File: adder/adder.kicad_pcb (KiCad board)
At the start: 2 copper layers, 52.9 x 21.5 mm, 29 parts

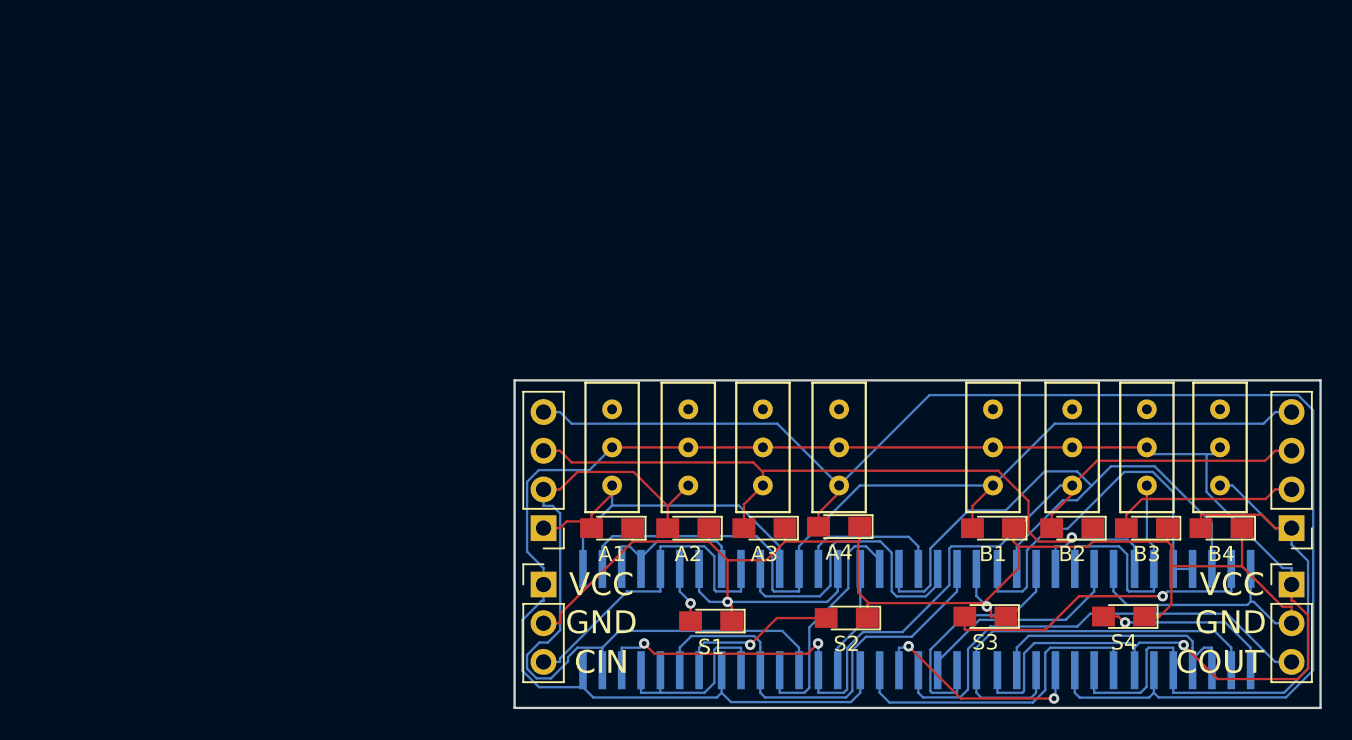
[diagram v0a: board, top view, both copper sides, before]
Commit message: Started on adder v3
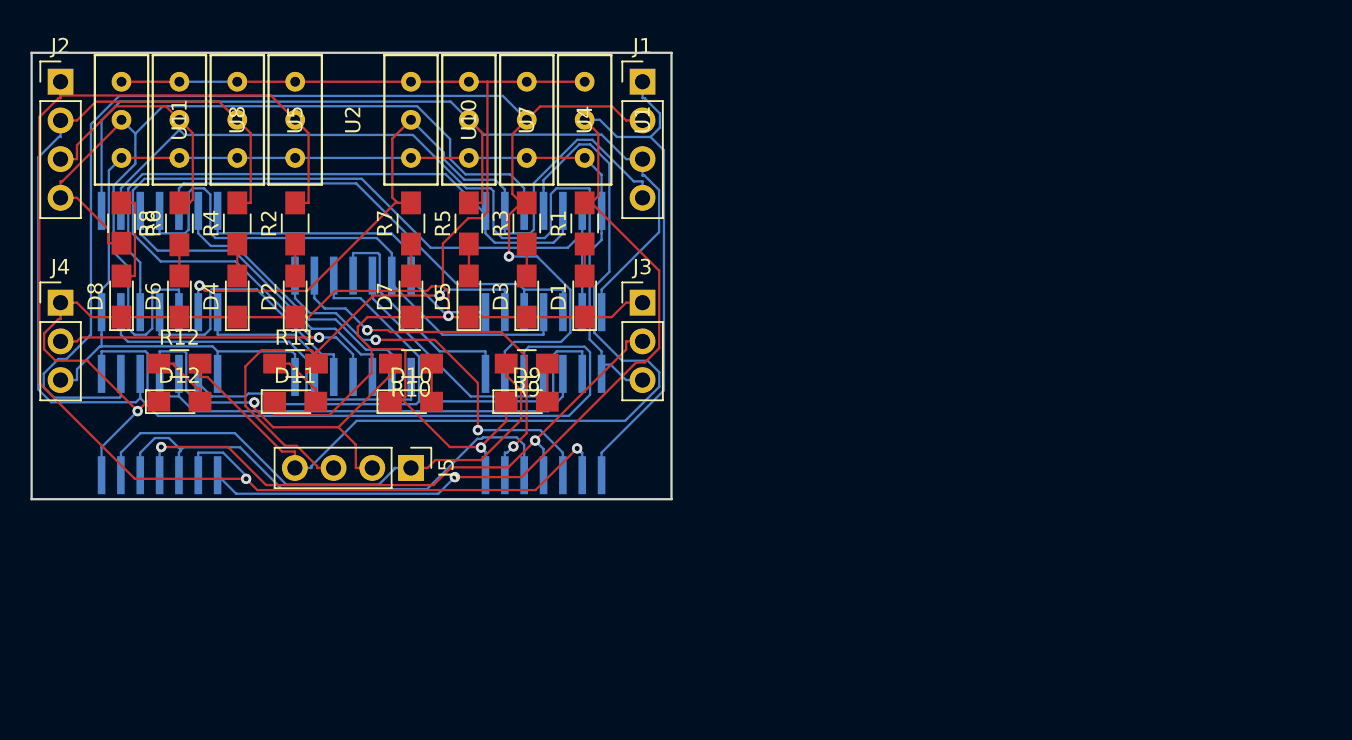
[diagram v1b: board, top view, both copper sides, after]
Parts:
- removed A1: LA1, LEDs:LED_0805_HandSoldering
- removed A1: A1, library:mini-vertical-slide-switch
- removed A2: LA2, LEDs:LED_0805_HandSoldering
- removed A2: A2, library:mini-vertical-slide-switch
- removed A3: LA3, LEDs:LED_0805_HandSoldering
- removed A3: A3, library:mini-vertical-slide-switch
- removed A4: A4, LEDs:LED_0805_HandSoldering
- removed A4: A4, library:mini-vertical-slide-switch
- removed AND (x2): AND, library:ssop14
- removed B1: LB1, LEDs:LED_0805_HandSoldering
- removed B1: B1, library:mini-vertical-slide-switch
- removed B2: LB2, LEDs:LED_0805_HandSoldering
- removed B2: B2, library:mini-vertical-slide-switch
- removed B3: LB3, LEDs:LED_0805_HandSoldering
- removed B3: B3, library:mini-vertical-slide-switch
- removed B4: LB4, LEDs:LED_0805_HandSoldering
- removed B4: B4, library:mini-vertical-slide-switch
- removed CIN: VIN, Pin_Headers:Pin_Header_Straight_1x03_Pitch2.54mm
- removed COUT: VOUT, Pin_Headers:Pin_Header_Straight_1x03_Pitch2.54mm
- removed OR: OR, library:ssop14
- removed S1: S1, LEDs:LED_0805_HandSoldering
- removed S2: S2, LEDs:LED_0805_HandSoldering
- removed S3: S3, LEDs:LED_0805_HandSoldering
- removed S4: S4, LEDs:LED_0805_HandSoldering
- removed VIN: A, Pin_Headers:Pin_Header_Straight_1x04_Pitch2.54mm
- removed VOUT: B, Pin_Headers:Pin_Header_Straight_1x04_Pitch2.54mm
- removed XOR (x2): XOR, library:ssop14
- added D1: A1, LEDs:LED_0805_HandSoldering, F.Cu at (134.4, 94.1)
- added D10: S2, LEDs:LED_0805_HandSoldering, F.Cu at (123.0, 101.0)
- added D11: S3, LEDs:LED_0805_HandSoldering, F.Cu at (115.4, 101.0)
- added D12: S4, LEDs:LED_0805_HandSoldering, F.Cu at (107.8, 101.0)
- added D2: B1, LEDs:LED_0805_HandSoldering, F.Cu at (115.4, 94.1)
- added D3: A2, LEDs:LED_0805_HandSoldering, F.Cu at (130.6, 94.1)
- added D4: B2, LEDs:LED_0805_HandSoldering, F.Cu at (111.6, 94.1)
- added D5: A3, LEDs:LED_0805_HandSoldering, F.Cu at (126.8, 94.1)
- added D6: B3, LEDs:LED_0805_HandSoldering, F.Cu at (107.8, 94.1)
- added D7: A4, LEDs:LED_0805_HandSoldering, F.Cu at (123.0, 94.1)
- added D8: B4, LEDs:LED_0805_HandSoldering, F.Cu at (104.0, 94.1)
- added D9: S1, LEDs:LED_0805_HandSoldering, F.Cu at (130.6, 101.0)
- added J1: AIN, Socket_Strips:Socket_Strip_Straight_1x04_Pitch2.54mm, F.Cu at (138.2, 80.0)
- added J2: BIN, Socket_Strips:Socket_Strip_Straight_1x04_Pitch2.54mm, F.Cu at (100.0, 80.0)
- added J3: VIN, Socket_Strips:Socket_Strip_Straight_1x03_Pitch2.54mm, F.Cu at (138.2, 94.5)
- added J4: VOUT, Socket_Strips:Socket_Strip_Straight_1x03_Pitch2.54mm, F.Cu at (100.0, 94.5)
- added J5: SOUT, Socket_Strips:Socket_Strip_Straight_1x04_Pitch2.54mm, F.Cu at (123.0, 105.3)
- added R1: R, Resistors_SMD:R_0805_HandSoldering, F.Cu at (134.4, 89.3)
- added R10: S2, Resistors_SMD:R_0805_HandSoldering, F.Cu at (123.0, 98.5)
- added R11: S3, Resistors_SMD:R_0805_HandSoldering, F.Cu at (115.4, 98.5)
- added R12: S4, Resistors_SMD:R_0805_HandSoldering, F.Cu at (107.8, 98.5)
- added R2: R, Resistors_SMD:R_0805_HandSoldering, F.Cu at (115.4, 89.3)
- added R3: R, Resistors_SMD:R_0805_HandSoldering, F.Cu at (130.6, 89.3)
- added R4: R, Resistors_SMD:R_0805_HandSoldering, F.Cu at (111.6, 89.3)
- added R5: R, Resistors_SMD:R_0805_HandSoldering, F.Cu at (126.8, 89.3)
- added R6: R, Resistors_SMD:R_0805_HandSoldering, F.Cu at (107.8, 89.3)
- added R7: R, Resistors_SMD:R_0805_HandSoldering, F.Cu at (123.0, 89.3)
- added R8: R, Resistors_SMD:R_0805_HandSoldering, F.Cu at (104.0, 89.3)
- added R9: S1, Resistors_SMD:R_0805_HandSoldering, F.Cu at (130.6, 98.5)
- added U1: A1, library:mini-vertical-slide-switch, F.Cu at (134.4, 82.5)
- added U10: A4, library:mini-vertical-slide-switch, F.Cu at (123.0, 82.5)
- added U11: B4, library:mini-vertical-slide-switch, F.Cu at (104.0, 82.5)
- added U12: AND, library:ssop14, B.Cu at (106.5, 91.8)
- added U13: OR, library:ssop14, B.Cu at (119.2, 96.0)
- added U2: B1, library:mini-vertical-slide-switch, F.Cu at (115.4, 82.5)
- added U3: XOR, library:ssop14, B.Cu at (106.5, 102.5)
- added U4: A2, library:mini-vertical-slide-switch, F.Cu at (130.6, 82.5)
- added U5: B2, library:mini-vertical-slide-switch, F.Cu at (111.6, 82.5)
- added U6: XOR, library:ssop14, B.Cu at (131.7, 91.8)
- added U7: A3, library:mini-vertical-slide-switch, F.Cu at (126.8, 82.5)
- added U8: B3, library:mini-vertical-slide-switch, F.Cu at (107.8, 82.5)
- added U9: AND, library:ssop14, B.Cu at (131.7, 102.5)
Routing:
- net VCC: track 132.8 -> 0.00 mm, vias 1 -> 0
- net +5V: track 0.00 -> 81.6 mm
- net /A1: track 26.5 -> 84.8 mm, vias 0 -> 1
- net /S4: track 12.0 -> 62.0 mm, vias 1 -> 0
- net GND: track 115.3 -> 164.9 mm, vias 2 -> 3
- net /A4: track 95.4 -> 51.0 mm, vias 0 -> 1
- net /XAB4: track 0.00 -> 41.8 mm
- net /COUT: track 31.2 -> 72.7 mm, vias 0 -> 1
- net /A2: track 49.7 -> 88.4 mm, vias 0 -> 1
- net /XAB2: track 0.00 -> 38.2 mm
- net /B3: track 29.7 -> 66.7 mm
- net /XAB1: track 0.00 -> 33.9 mm
- net /XAB3: track 0.00 -> 32.7 mm
- net /S1: track 3.72 -> 35.6 mm, vias 1 -> 0
- net /B1: track 59.9 -> 89.9 mm, vias 0 -> 2
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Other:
- board size 52.9 x 21.5 mm -> 42 x 29.3 mm
- board text removed: "CIN"
- board text removed: "COUT"
- board text removed: "GND"
- board text removed: "VCC"
